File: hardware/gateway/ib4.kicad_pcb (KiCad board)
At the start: 4 copper layers, 68.4 x 55.7 mm, 7 parts, among them J1 Conn_01x12_Female, J2 Conn_01x09_Female

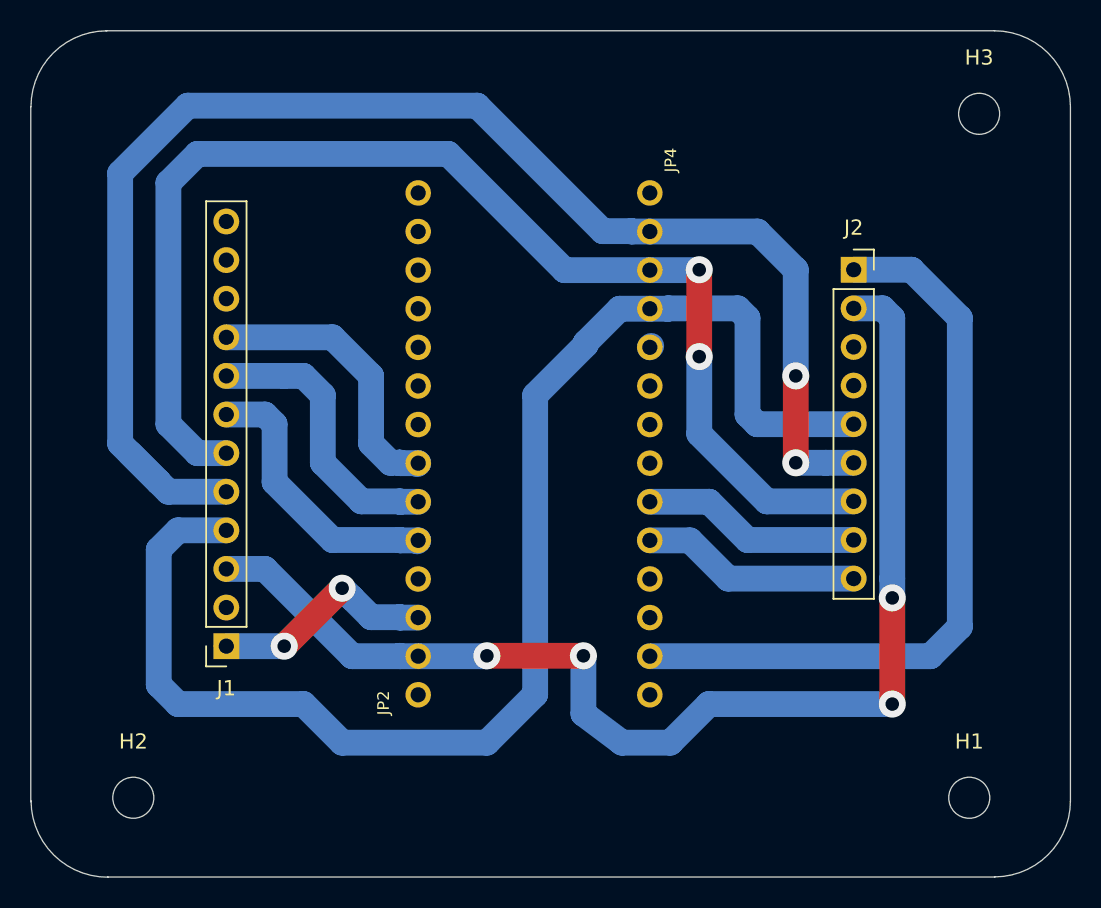
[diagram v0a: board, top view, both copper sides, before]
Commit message: update
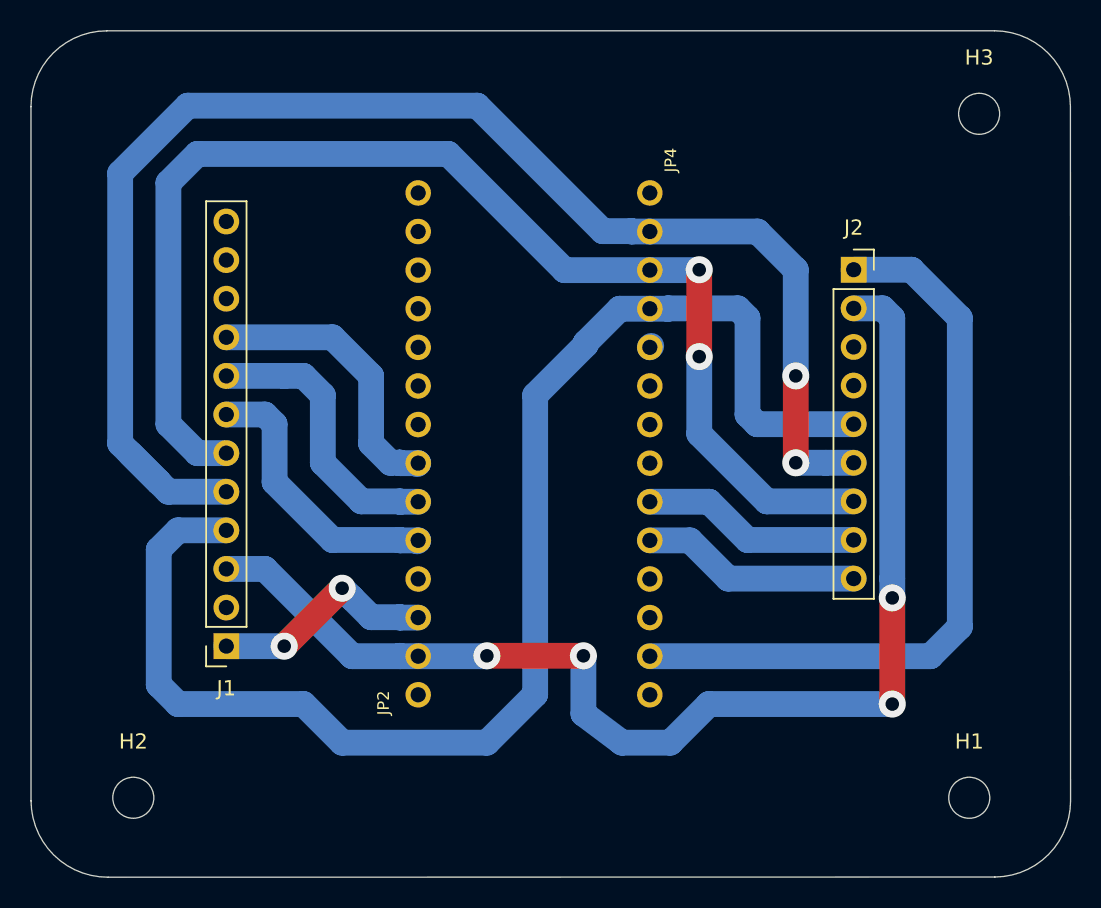
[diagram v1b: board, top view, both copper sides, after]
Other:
- outline, holes or cut-outs redrawn
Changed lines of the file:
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@@
       (drillshape 0)
       (scaleselection 1)
-      (outputdirectory "milling/"))
+      (outputdirectory "gerb/"))
   )
   (net 0 "")
@@
     (pad 1 np_thru_hole circle (at 0 0) (size 2.7 2.7) (drill 2.7) (layers *.Cu *.Mask))
   )
-  (gr_line (start 126.6571 37.5539) (end 126.6571 83.235945) (layer Edge.Cuts) (width 0.05))
-  (gr_line (start 58.2549 37.5412) (end 58.2549 83.2612) (layer Edge.Cuts) (width 0.05))
-  (gr_line (start 121.6914 88.2142) (end 63.3095 88.2142) (layer Edge.Cuts) (width 0.05))
-  (gr_line (start 63.1952 32.5374) (end 121.666 32.5374) (layer Edge.Cuts) (width 0.05))
+  (gr_line (start 126.6571 37.5539) (end 126.665223 83.2104) (layer Edge.Cuts) (width 0.05))
+  (gr_line (start 58.2676 37.5285) (end 58.271533 83.204433) (layer Edge.Cuts) (width 0.05))
+  (gr_line (start 121.6914 88.2142) (end 63.3476 88.2269) (layer Edge.Cuts) (width 0.05))
+  (gr_line (start 63.253834 32.542266) (end 121.666 32.5374) (layer Edge.Cuts) (width 0.05))
   (gr_arc (start 63.3208 83.177633) (end 58.271533 83.204433) (angle -90) (layer Edge.Cuts) (width 0.05))
-  (gr_arc (start 121.661333 83.2104) (end 121.661333 88.206167) (angle -90) (layer Edge.Cuts) (width 0.05))
-  (gr_arc (start 121.653155 37.541345) (end 126.6571 37.541345) (angle -90) (layer Edge.Cuts) (width 0.05))
+  (gr_arc (start 121.661333 83.2104) (end 121.6914 88.2142) (angle -89.65572336) (layer Edge.Cuts) (width 0.05))
+  (gr_arc (start 121.653155 37.541345) (end 126.6571 37.5539) (angle -89.99667949) (layer Edge.Cuts) (width 0.05))
   (gr_arc (start 63.253834 37.5285) (end 63.253834 32.542266) (angle -90) (layer Edge.Cuts) (width 0.05))
   (segment (start 99.0753 53.2739) (end 98.9838 53.3654) (width 1.7) (layer Bottom) (net 0) (status 30))
